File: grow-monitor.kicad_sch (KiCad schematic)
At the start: 68 parts, among them J1 PH 2.0, J2 I2C1, J3 DS18B20, M1 M5StampS3, M2 AHT21B, P1 PCB_Patch, Q1 AO3401A, Q2 ALS-PT19-315C, Q3 AO3401A, Q4 2N7002, SW1 PWR2, SW2 CALIB, SW3 EN, SW4 PROG, SW5 KILL, SW6 PWR1, T1 Tooling, U1 SPX3819M5-L-3-3, U2 TPL5110, U4 DS18B20, U5 NE555P

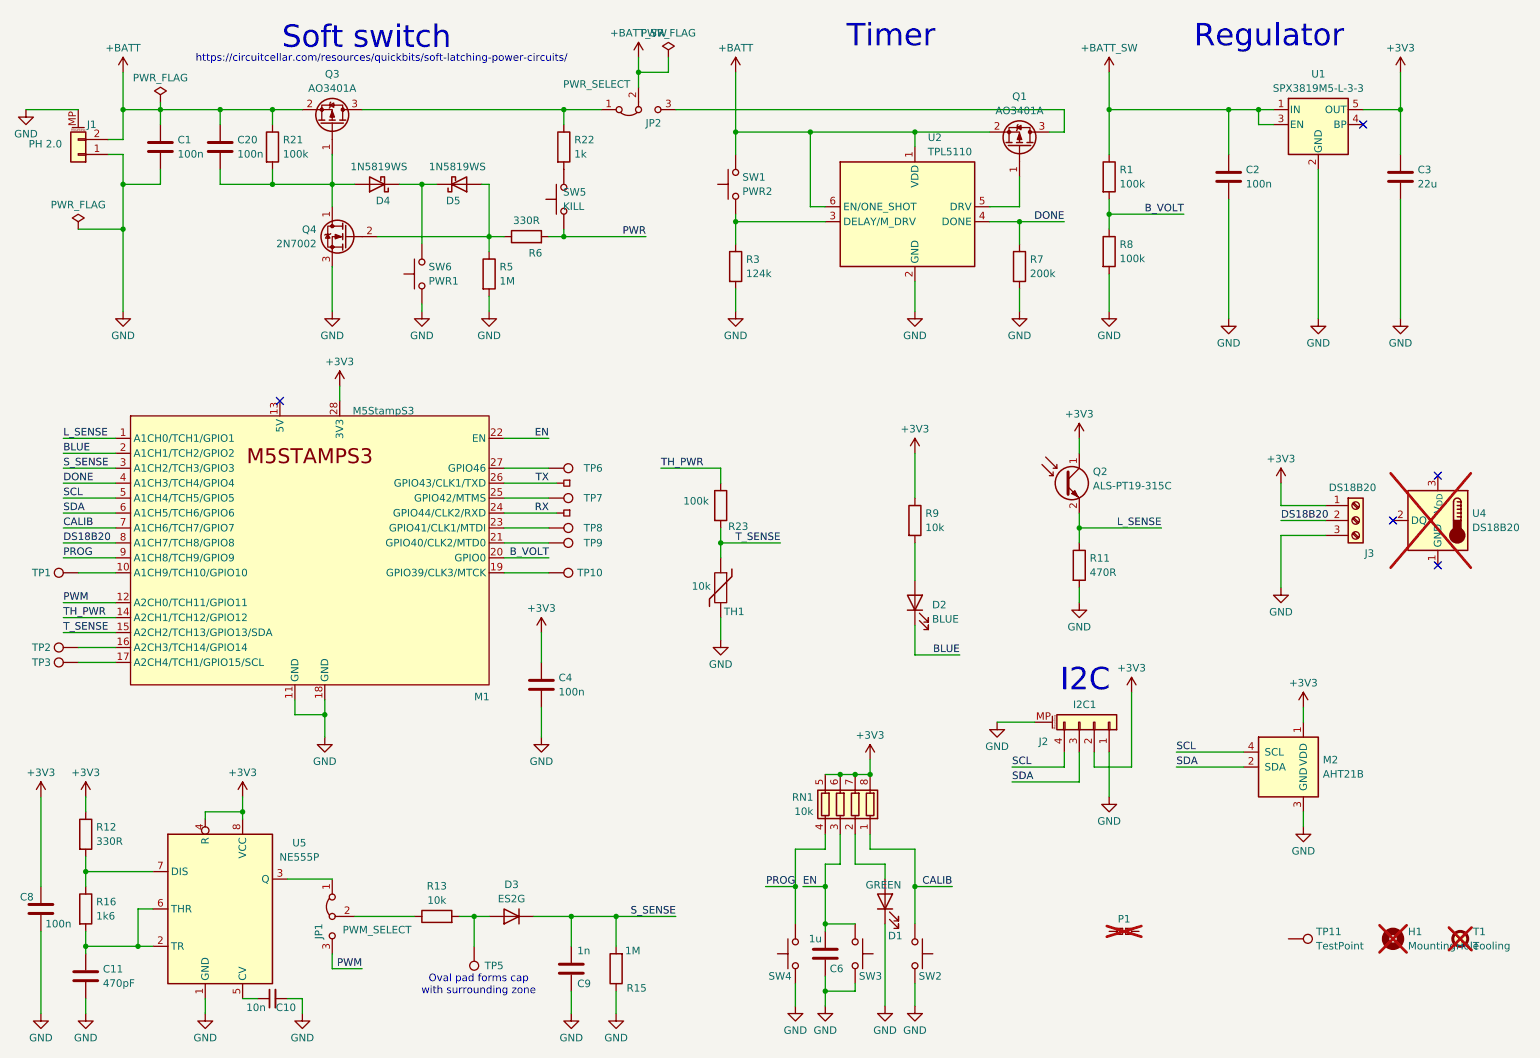
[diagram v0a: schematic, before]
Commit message: More improvements
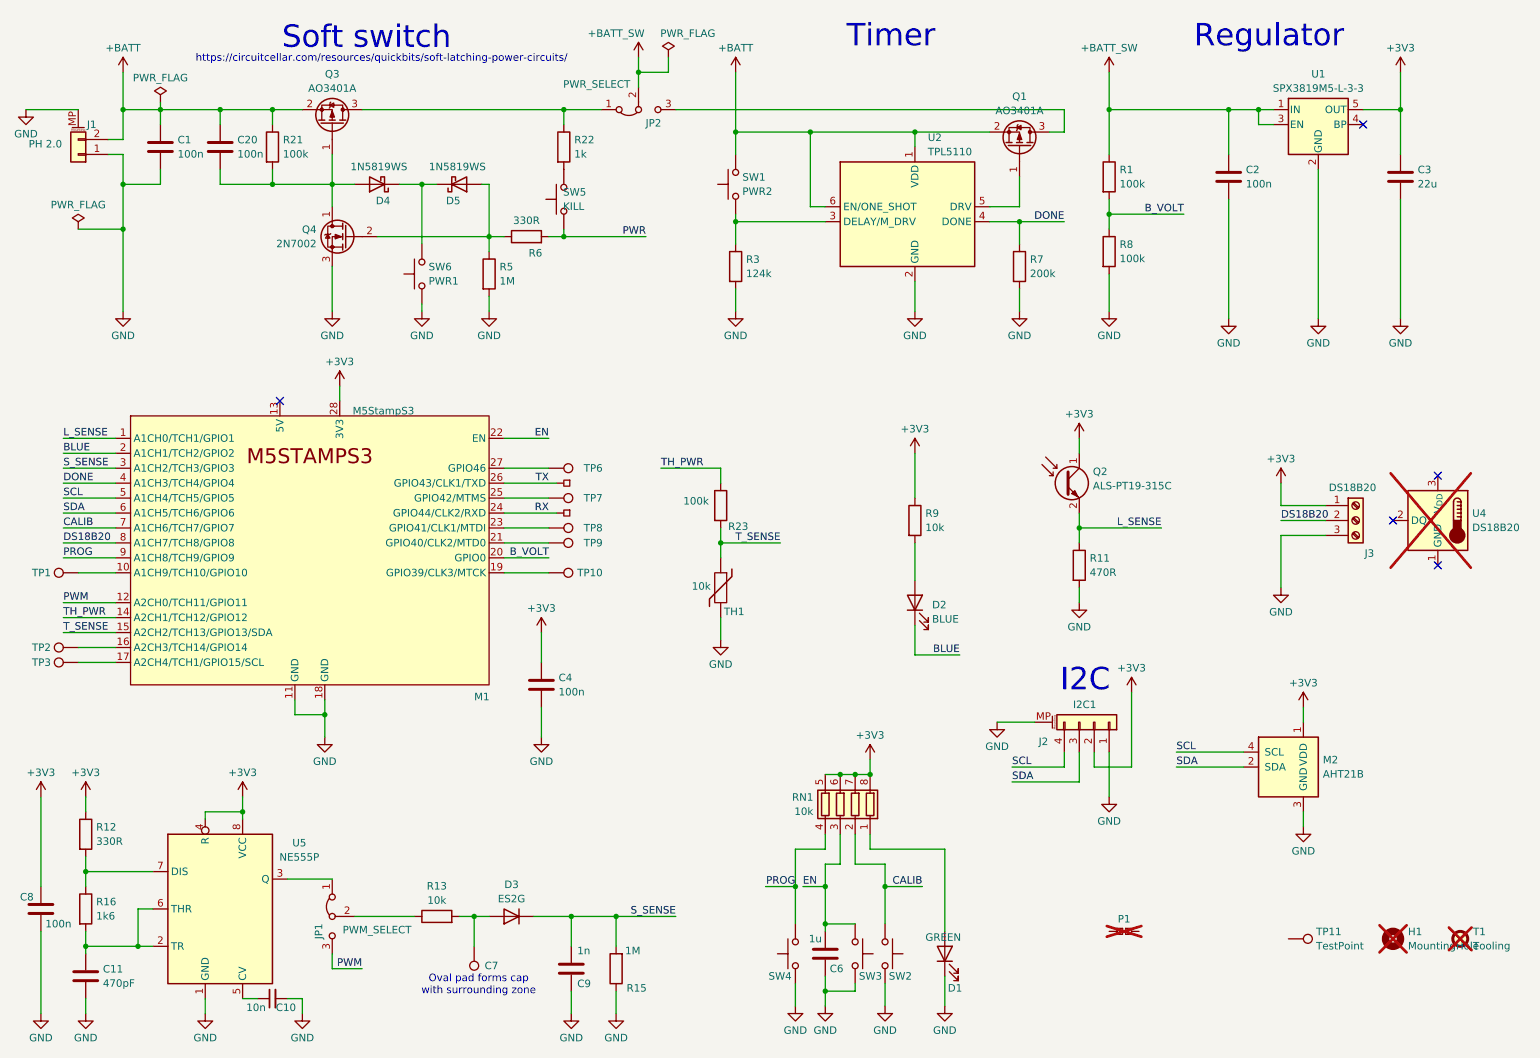
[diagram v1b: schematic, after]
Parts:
- JP5, JP6, TP1, TP10, TP11, TP2, TP3, TP6, TP7, TP8, TP9: footprint TestPoint:TestPoint_Pad_1.0x1.0mm -> local:TestPoint_Pad_1.0x1.0mm
- renumbered TP5 to C7
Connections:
- net CALIB: now also RN1.2 (R2.1); no longer RN1.1 (R1.1)
- net at D1.2 (A): now also RN1.1 (R1.1); no longer RN1.2 (R2.1)
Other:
- moved on the sheet: D1, SW2
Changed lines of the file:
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@@
 	)
 	(junction
-		(at 135.89 38.1)
+		(at 161.29 166.37)
 		(diameter 0)
 		(color 0 0 0 0)
 	)
 	(junction
-		(at 31.75 54.61)
+		(at 135.89 38.1)
 		(diameter 0)
 		(color 0 0 0 0)
 	)
 	(junction
-		(at 184.15 53.34)
+		(at 31.75 54.61)
 		(diameter 0)
 		(color 0 0 0 0)
 	)
 	(junction
-		(at 166.37 166.37)
+		(at 184.15 53.34)
 		(diameter 0)
 		(color 0 0 0 0)
@@
 	(wire
 		(pts
-			(xy 161.29 162.56) (xy 161.29 165.1)
+			(xy 171.45 160.02) (xy 171.45 173.99)
 		)
 		(stroke
@@
 	(wire
 		(pts
-			(xy 166.37 160.02) (xy 166.37 166.37)
-		)
-		(stroke
-			(width 0)
-			(type default)
-		)
-	)
-	(wire
-		(pts
 			(xy 151.13 50.8) (xy 148.59 50.8)
 		)
@@
 	(wire
 		(pts
-			(xy 166.37 182.88) (xy 166.37 186.69)
+			(xy 161.29 182.88) (xy 161.29 186.69)
 		)
 		(stroke
@@
 	(wire
 		(pts
-			(xy 166.37 166.37) (xy 172.72 166.37)
+			(xy 161.29 166.37) (xy 167.64 166.37)
 		)
 		(stroke
@@
 	(wire
 		(pts
-			(xy 158.75 160.02) (xy 166.37 160.02)
-		)
-		(stroke
-			(width 0)
-			(type default)
-		)
-	)
-	(wire
-		(pts
 			(xy 151.13 184.15) (xy 151.13 186.69)
 		)
@@
 	(wire
 		(pts
-			(xy 166.37 166.37) (xy 166.37 172.72)
+			(xy 161.29 162.56) (xy 161.29 166.37)
 		)
 		(stroke
@@
 	(wire
 		(pts
-			(xy 161.29 172.72) (xy 161.29 186.69)
+			(xy 171.45 181.61) (xy 171.45 186.69)
 		)
 		(stroke
@@
 	(wire
 		(pts
+			(xy 161.29 166.37) (xy 161.29 172.72)
+		)
+		(stroke
+			(width 0)
+			(type default)
+		)
+	)
+	(wire
+		(pts
 			(xy 194.31 143.51) (xy 194.31 148.59)
 		)
@@
 	(wire
 		(pts
+			(xy 171.45 160.02) (xy 158.75 160.02)
+		)
+		(stroke
+			(width 0)
+			(type default)
+		)
+	)
+	(wire
+		(pts
 			(xy 93.98 55.88) (xy 93.98 58.42)
 		)
@@
 	)
 	(label "CALIB"
-		(at 172.72 166.37 180)
+		(at 167.64 166.37 180)
 		(fields_autoplaced yes)
 		(effects
@@
 			)
 		)
-		(property "Footprint" "TestPoint:TestPoint_Pad_1.0x1.0mm"
+		(property "Footprint" "local:TestPoint_Pad_1.0x1.0mm"
 			(at 109.22 107.95 0)
 			(effects
@@
 	(symbol
 		(lib_id "power:GND")
-		(at 161.29 186.69 0)
+		(at 171.45 186.69 0)
 		(unit 1)
 		(exclude_from_sim no)
@@
 		(fields_autoplaced yes)
 		(property "Reference" "#PWR026"
-			(at 161.29 193.04 0)
+			(at 171.45 193.04 0)
 			(effects
 				(font
@@
 		)
 		(property "Value" "GND"
-			(at 161.29 190.8231 0)
+			(at 171.45 190.8231 0)
 			(effects
 				(font
@@
 		)
 		(property "Footprint" ""
-			(at 161.29 186.69 0)
+			(at 171.45 186.69 0)
 			(effects
 				(font
@@
 		)
 		(property "Datasheet" ""
-			(at 161.29 186.69 0)
+			(at 171.45 186.69 0)
 			(effects
 				(font
@@
 		)
 		(property "Description" "Power symbol creates a global label with name \"GND\" , ground"
-			(at 161.29 186.69 0)
+			(at 171.45 186.69 0)
 			(effects
 				(font
@@
 			)
 		)
-		(property "Footprint" "TestPoint:TestPoint_Pad_1.0x1.0mm"
+		(property "Footprint" "local:TestPoint_Pad_1.0x1.0mm"
 			(at 19.05 125.73 0)
 			(effects
@@
 			)
 		)
-		(property "Footprint" "TestPoint:TestPoint_Pad_1.0x1.0mm"
+		(property "Footprint" "local:TestPoint_Pad_1.0x1.0mm"
 			(at 19.05 128.27 0)
 			(effects
@@
 			)
 		)
-		(property "Footprint" "TestPoint:TestPoint_Pad_1.0x1.0mm"
+		(property "Footprint" "local:TestPoint_Pad_1.0x1.0mm"
 			(at 107.95 102.87 0)
 			(effects
@@
 		(exclude_from_sim no)
 		(in_bom yes)
-		(on_board yes)
+		(on_board no)
 		(dnp no)
 		(fields_autoplaced yes)
@@
 			)
 		)
-		(property "Footprint" "TestPoint:TestPoint_Pad_1.0x1.0mm"
+		(property "Footprint" "local:TestPoint_Pad_1.0x1.0mm"
 			(at 234.95 175.26 0)
 			(effects
@@
 	(symbol
 		(lib_id "Switch:SW_Push")
-		(at 166.37 177.8 270)
+		(at 161.29 177.8 270)
 		(mirror x)
 		(unit 1)
@@
 		(dnp no)
 		(property "Reference" "SW2"
-			(at 170.942 181.61 90)
+			(at 165.862 181.61 90)
 			(effects
 				(font
@@
 		)
 		(property "Value" "CALIB"
-			(at 165.227 179.0121 90)
+			(at 160.147 179.0121 90)
 			(effects
 				(font
@@
 		)
 		(property "Footprint" "local:SW_Push_SPST_NO_432"
-			(at 171.45 177.8 0)
+			(at 166.37 177.8 0)
 			(effects
 				(font
@@
 		)
 		(property "Datasheet" "~"
-			(at 171.45 177.8 0)
+			(at 166.37 177.8 0)
 			(effects
 				(font
@@
 		)
 		(property "Description" "Push button switch, generic, two pins"
-			(at 166.37 177.8 0)
+			(at 161.29 177.8 0)
 			(effects
 				(font
@@
 		)
 		(property "LCSC" "C707339"
-			(at 166.37 177.8 0)
+			(at 161.29 177.8 0)
 			(effects
 				(font
@@
 	(symbol
 		(lib_id "Device:LED")
-		(at 161.29 168.91 90)
+		(at 171.45 177.8 90)
 		(unit 1)
 		(exclude_from_sim no)
@@
 		(dnp no)
 		(property "Reference" "D1"
-			(at 161.798 174.752 90)
+			(at 171.958 183.642 90)
 			(effects
 				(font
@@
 		)
 		(property "Value" "GREEN"
-			(at 157.988 166.116 90)
+			(at 168.148 175.006 90)
 			(effects
 				(font
@@
 		)
 		(property "Footprint" "LED_SMD:LED_0603_1608Metric"
-			(at 161.29 168.91 0)
+			(at 171.45 177.8 0)
 			(effects
 				(font
@@
 		)
 		(property "Datasheet" "~"
-			(at 161.29 168.91 0)
+			(at 171.45 177.8 0)
 			(effects
 				(font
@@
 		)
 		(property "Description" "Light emitting diode"
-			(at 161.29 168.91 0)
+			(at 171.45 177.8 0)
 			(effects
 				(font
@@
 		)
 		(property "LCSC" ""
-			(at 161.29 168.91 0)
+			(at 171.45 177.8 0)
 			(effects
 				(font
@@
 			)
 		)
-		(property "Footprint" "TestPoint:TestPoint_Pad_1.0x1.0mm"
+		(property "Footprint" "local:TestPoint_Pad_1.0x1.0mm"
 			(at 19.05 113.03 0)
 			(effects
@@
 		(on_board yes)
 		(dnp no)
-		(fields_autoplaced yes)
 		(property "Reference" "#PWR019"
 			(at 119.38 29.21 0)
@@
 		)
 		(property "Value" "+BATT_SW"
-			(at 119.38 21.2669 0)
+			(at 115.57 21.336 0)
 			(effects
 				(font
@@
 			)
 		)
-		(property "Footprint" "TestPoint:TestPoint_Pad_1.0x1.0mm"
+		(property "Footprint" "local:TestPoint_Pad_1.0x1.0mm"
 			(at 109.22 95.25 0)
 			(effects
@@
 			)
 		)
-		(property "Footprint" "TestPoint:TestPoint_Pad_1.0x1.0mm"
+		(property "Footprint" "local:TestPoint_Pad_1.0x1.0mm"
 			(at 109.22 113.03 0)
 			(effects
@@
 			)
 		)
-		(property "Footprint" "TestPoint:TestPoint_Pad_1.0x1.0mm"
+		(property "Footprint" "local:TestPoint_Pad_1.0x1.0mm"
 			(at 109.22 105.41 0)
 			(effects
@@
 			)
 		)
-		(property "Footprint" "TestPoint:TestPoint_Pad_1.0x1.0mm"
+		(property "Footprint" "local:TestPoint_Pad_1.0x1.0mm"
 			(at 107.95 97.79 0)
 			(effects
@@
 	(symbol
 		(lib_id "power:GND")
-		(at 166.37 186.69 0)
+		(at 161.29 186.69 0)
 		(unit 1)
 		(exclude_from_sim no)
@@
 		(fields_autoplaced yes)
 		(property "Reference" "#PWR029"
-			(at 166.37 193.04 0)
+			(at 161.29 193.04 0)
 			(effects
 				(font
@@
 		)
 		(property "Value" "GND"
-			(at 166.37 190.8231 0)
+			(at 161.29 190.8231 0)
 			(effects
 				(font
@@
 		)
 		(property "Footprint" ""
-			(at 166.37 186.69 0)
+			(at 161.29 186.69 0)
 			(effects
 				(font
@@
 		)
 		(property "Datasheet" ""
-			(at 166.37 186.69 0)
+			(at 161.29 186.69 0)
 			(effects
 				(font
@@
 		)
 		(property "Description" "Power symbol creates a global label with name \"GND\" , ground"
-			(at 166.37 186.69 0)
+			(at 161.29 186.69 0)
 			(effects
 				(font
@@
 		(on_board yes)
 		(dnp no)
-		(fields_autoplaced yes)
 		(property "Reference" "#FLG03"
 			(at 124.46 23.495 0)
@@
 		)
 		(property "Value" "PWR_FLAG"
-			(at 124.46 21.2669 0)
+			(at 127.762 21.336 0)
 			(effects
 				(font
@@
 		(on_board yes)
 		(dnp no)
-		(property "Reference" "TP5"
+		(property "Reference" "C7"
 			(at 93.218 179.832 90)
 			(effects
@@
 			(project "grow-monitor"
 				(path "/ff355f4c-e562-4fd3-bc17-978a5d849f6b"
-					(reference "TP5")
+					(reference "C7")
 					(unit 1)
 				)
@@
 			)
 		)
-		(property "Footprint" "TestPoint:TestPoint_Pad_1.0x1.0mm"
+		(property "Footprint" "local:TestPoint_Pad_1.0x1.0mm"
 			(at 109.22 100.33 0)
 			(effects
